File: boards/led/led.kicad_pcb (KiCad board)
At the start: 2 copper layers, 20 x 20 mm, 2 parts, among them J1 RJ45

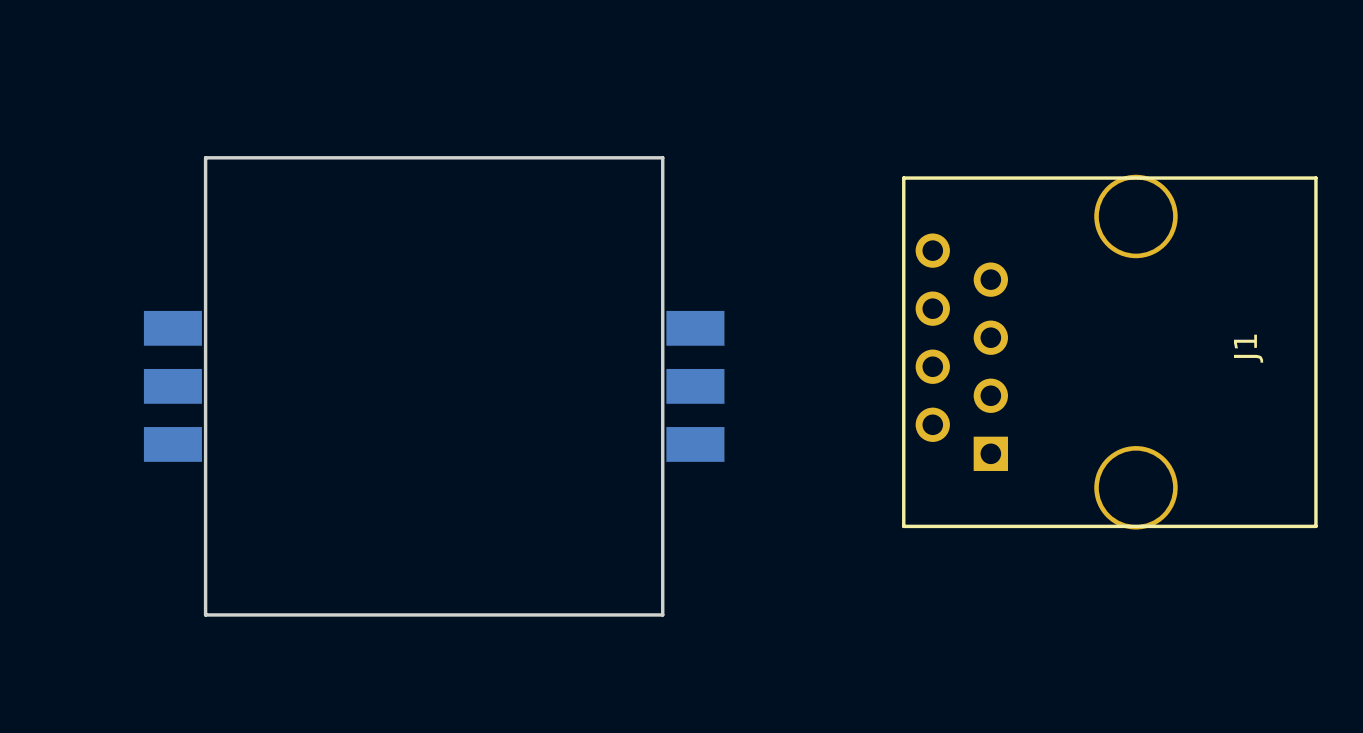
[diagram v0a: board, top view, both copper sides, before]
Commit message: led pcb
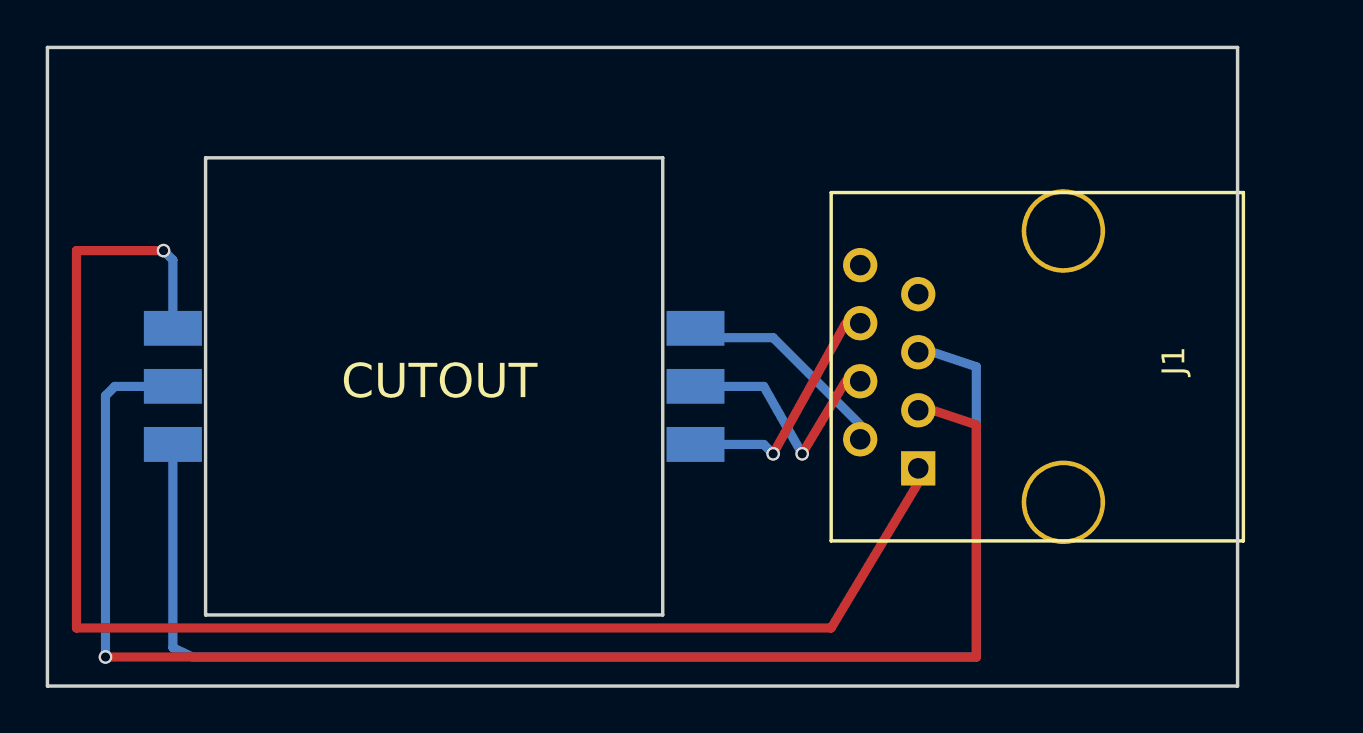
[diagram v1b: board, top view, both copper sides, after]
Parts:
- moved J1 3.24 mm to (176.5, 104.1)
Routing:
- net Net-(D1-Pad2): track 0.00 -> 65.5 mm, vias 0 -> 1
- net Net-(D1-Pad1): track 0.00 -> 65.0 mm, vias 0 -> 1
- net Net-(D1-Pad3): track 0.00 -> 59.5 mm
- net Net-(D1-Pad4): track 0.00 -> 11.2 mm, vias 0 -> 1
- net Net-(D1-Pad5): track 0.00 -> 10.7 mm, vias 0 -> 1
- net Net-(D1-Pad6): track 0.00 -> 9.59 mm
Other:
- board size 20 x 20 mm -> 52.1 x 27.9 mm
- net class Default: clearance 0.4 -> 0.2; trace_width 0.25 -> 0.4
- rule trace_clearance: 0.4 -> 0.2
- board text added: "CUTOUT"
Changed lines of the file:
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@@
   (general
     (links 6)
-    (no_connects 6)
-    (area 0 0 0 0)
+    (no_connects 0)
+    (area 132.004999 90.094999 184.729001 118.185001)
     (thickness 1.6)
-    (drawings 4)
-    (tracks 0)
+    (drawings 9)
+    (tracks 38)
     (zones 0)
     (modules 2)
@@
   )
   (setup
-    (last_trace_width 0.25)
-    (trace_clearance 0.4)
+    (last_trace_width 0.4)
+    (trace_clearance 0.2)
     (zone_clearance 0.508)
     (zone_45_only yes)
@@
   (net 8 "Net-(J1-Pad8)")
   (net_class Default "This is the default net class."
-    (clearance 0.4)
-    (trace_width 0.25)
+    (clearance 0.2)
+    (trace_width 0.4)
     (via_dia 0.6)
     (via_drill 0.4)
@@
   )
   (module Connect:RJ45_8 (layer F.Cu)
-    (at 179.705 103.505 90)
+    (at 176.53 104.14 90)
     (tags RJ45)
     (fp_text reference J1 (at 0.254 4.826 90) (layer F.SilkS)
@@
     )
   )
+  (gr_line (start 132.08 118.11) (end 184.15 118.11) (angle 90) (layer Edge.Cuts) (width 0.15))
+  (gr_line (start 132.08 90.17) (end 132.08 118.11) (angle 90) (layer Edge.Cuts) (width 0.15))
+  (gr_line (start 184.15 90.17) (end 132.08 90.17) (angle 90) (layer Edge.Cuts) (width 0.15))
+  (gr_line (start 184.15 118.11) (end 184.15 90.17) (angle 90) (layer Edge.Cuts) (width 0.15))
+  (gr_text CUTOUT (at 149.225 104.775) (layer F.SilkS)
+    (effects (font (size 1.5 1.5) (thickness 0.3)))
+  )
   (gr_line (start 139 115) (end 139 95) (angle 90) (layer Edge.Cuts) (width 0.15))
   (gr_line (start 159 115) (end 139 115) (angle 90) (layer Edge.Cuts) (width 0.15))
   (gr_line (start 159 95) (end 159 115) (angle 90) (layer Edge.Cuts) (width 0.15))
   (gr_line (start 139 95) (end 159 95) (angle 90) (layer Edge.Cuts) (width 0.15))
+  (segment (start 170.18 106.045) (end 170.815 106.045) (width 0.25) (layer F.Cu) (net 1) (status 30))
+  (segment (start 170.815 106.045) (end 172.72 106.68) (width 0.4) (layer F.Cu) (net 1) (status 10))
+  (segment (start 172.72 106.68) (end 172.72 116.84) (width 0.4) (layer F.Cu) (net 1))
+  (segment (start 172.72 116.84) (end 134.62 116.84) (width 0.4) (layer F.Cu) (net 1))
+  (via (at 134.62 116.84) (size 0.6) (drill 0.4) (layers F.Cu B.Cu) (net 1))
+  (segment (start 134.62 116.84) (end 134.62 105.41) (width 0.4) (layer B.Cu) (net 1))
+  (segment (start 134.62 105.41) (end 135.03 105) (width 0.4) (layer B.Cu) (net 1))
+  (segment (start 135.03 105) (end 137.57 105) (width 0.4) (layer B.Cu) (net 1))
+  (segment (start 170.18 103.505) (end 170.815 103.505) (width 0.25) (layer B.Cu) (net 2) (status 30))
+  (segment (start 170.815 103.505) (end 172.72 104.14) (width 0.4) (layer B.Cu) (net 2) (status 10))
+  (segment (start 172.72 104.14) (end 172.72 116.84) (width 0.4) (layer B.Cu) (net 2))
+  (segment (start 172.72 116.84) (end 138.43 116.84) (width 0.4) (layer B.Cu) (net 2))
+  (segment (start 138.43 116.84) (end 137.57 116.43) (width 0.4) (layer B.Cu) (net 2))
+  (segment (start 137.57 116.43) (end 137.57 107.54) (width 0.4) (layer B.Cu) (net 2))
+  (segment (start 137.57 99.47) (end 137.57 102.46) (width 0.4) (layer B.Cu) (net 3))
+  (segment (start 137.16 99.06) (end 137.57 99.47) (width 0.4) (layer B.Cu) (net 3))
+  (via (at 137.16 99.06) (size 0.6) (drill 0.4) (layers F.Cu B.Cu) (net 3))
+  (segment (start 133.35 99.06) (end 137.16 99.06) (width 0.4) (layer F.Cu) (net 3))
+  (segment (start 133.35 102.87) (end 133.35 99.06) (width 0.4) (layer F.Cu) (net 3))
+  (segment (start 170.18 109.22) (end 166.37 115.57) (width 0.4) (layer F.Cu) (net 3) (status 10))
+  (segment (start 166.37 115.57) (end 133.35 115.57) (width 0.4) (layer F.Cu) (net 3))
+  (segment (start 133.35 115.57) (end 133.35 102.87) (width 0.4) (layer F.Cu) (net 3))
+  (segment (start 170.18 108.585) (end 170.18 109.22) (width 0.25) (layer F.Cu) (net 3) (status 30))
+  (segment (start 167.64 107.315) (end 167.64 106.68) (width 0.25) (layer B.Cu) (net 4) (status 10))
+  (segment (start 163.83 102.87) (end 160.84 102.87) (width 0.4) (layer B.Cu) (net 4))
+  (segment (start 167.64 106.68) (end 163.83 102.87) (width 0.4) (layer B.Cu) (net 4))
+  (segment (start 160.84 102.87) (end 160.43 102.46) (width 0.25) (layer B.Cu) (net 4))
+  (segment (start 167.64 104.775) (end 167.005 104.775) (width 0.25) (layer F.Cu) (net 5) (status 30))
+  (segment (start 167.005 104.775) (end 165.1 107.95) (width 0.4) (layer F.Cu) (net 5) (status 10))
+  (via (at 165.1 107.95) (size 0.6) (drill 0.4) (layers F.Cu B.Cu) (net 5))
+  (segment (start 165.1 107.95) (end 163.42 105) (width 0.4) (layer B.Cu) (net 5))
+  (segment (start 163.42 105) (end 160.43 105) (width 0.4) (layer B.Cu) (net 5))
+  (segment (start 167.64 102.235) (end 167.005 102.235) (width 0.25) (layer F.Cu) (net 6) (status 30))
+  (segment (start 167.005 102.235) (end 163.83 107.95) (width 0.4) (layer F.Cu) (net 6) (status 10))
+  (segment (start 163.42 107.54) (end 160.43 107.54) (width 0.4) (layer B.Cu) (net 6))
+  (segment (start 163.83 107.95) (end 163.42 107.54) (width 0.4) (layer B.Cu) (net 6))
+  (via (at 163.83 107.95) (size 0.6) (drill 0.4) (layers F.Cu B.Cu) (net 6))
+  (segment (start 160.88 107.54) (end 160.43 107.54) (width 0.25) (layer B.Cu) (net 6))
   (zone (net 0) (net_name "") (layer F.Cu) (hatch edge 0.508)
     (connect_pads (clearance 0.508))
